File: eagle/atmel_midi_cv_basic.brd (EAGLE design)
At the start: 100 x 80 mm, 46 parts, among them IC1 TL072P, IC2 TL072P, U1 ATMEGA328P_PDIP

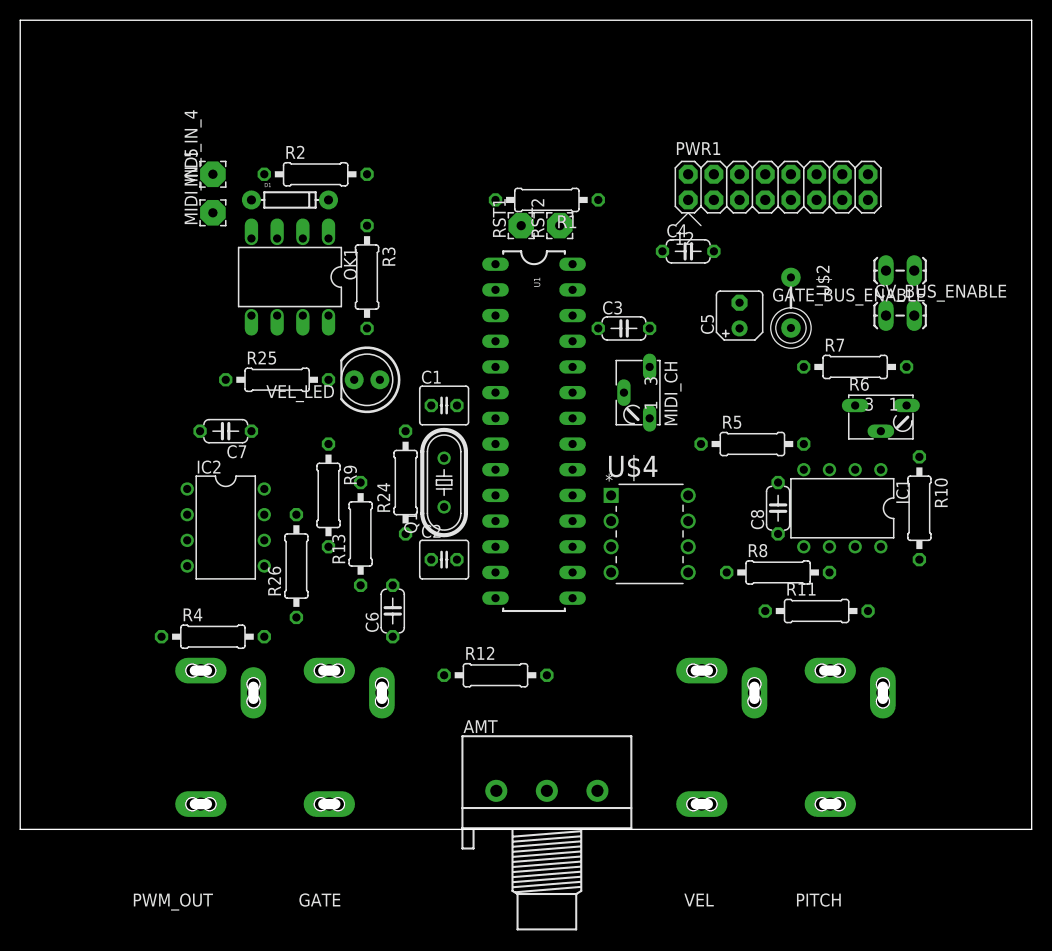
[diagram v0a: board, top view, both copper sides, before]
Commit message: possible route
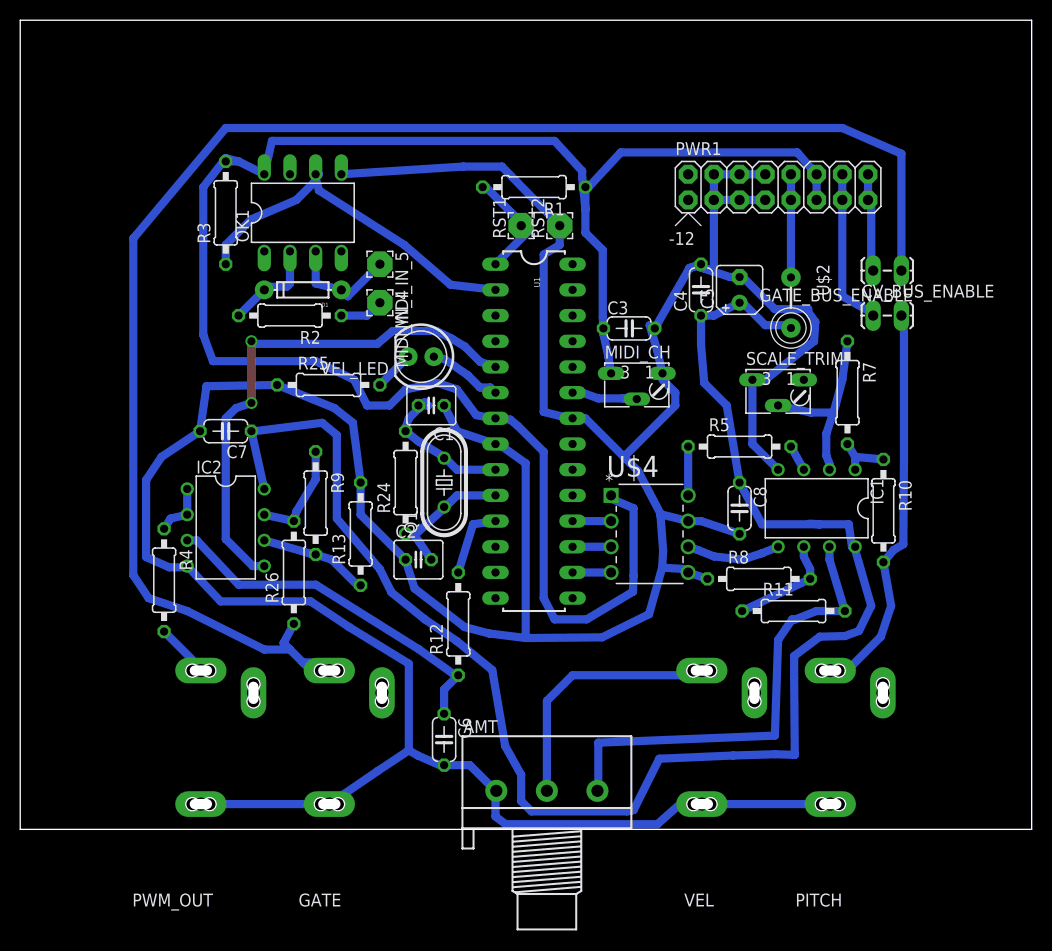
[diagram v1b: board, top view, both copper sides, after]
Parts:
- removed R6: 10k, pot:B64W
- added SCALE_TRIM: 10k, pot:B64W
- moved MIDI_IN_4 20.8 mm to (35.6, 52.1), turned to 270 degrees
- moved MIDI_IN_5 17.3 mm to (35.6, 55.9), turned to 270 degrees
- moved R3 15.3 mm to (20.3, 61.0), turned to 90 degrees
- moved R2 14.2 mm to (26.7, 50.8), turned to 180 degrees
- moved C6 13.7 mm to (41.9, 8.89), turned to 270 degrees
- moved D1 8.98 mm to (27.9, 53.3), turned to 180 degrees
- moved R4 7.38 mm to (14.2, 24.6), turned to 270 degrees
- moved OK1 6.48 mm to (27.9, 61.0), turned to 0 degrees
- moved R12 6.27 mm to (43.3, 20.3), turned to 90 degrees
- moved VEL_LED 5.80 mm to (39.6, 46.7)
- moved R25 5.11 mm to (30.5, 43.9)
- moved C4 4.02 mm to (67.3, 53.3), turned to 90 degrees
- moved C8 3.81 mm to (71.1, 31.8), turned to 270 degrees
- moved R10 3.57 mm to (85.3, 31.5)
- moved R7 2.65 mm to (81.8, 43.2), turned to 270 degrees
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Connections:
- removed net GND: AMT.1, C1.1, C2.1, C3.2, C4.2, C5.-, C6.2, C7.2, C8.2, GATE.P$1, IC1.4, IC2.4, MIDI_CH.E, OK1.5, PITCH.P$1, PWM_OUT.P$1, PWR1.3, PWR1.4, PWR1.5, PWR1.6, PWR1.7, PWR1.8, R13.2, R25.1, R6.E, R8.1, RST2.1, U$4.5, U$4.7, U1.22, U1.8, VEL.P$1
- new net N$29: AMT.1, C1.1, C2.1, C3.2, C4.2, C5.-, C6.2, C7.2, C8.2, GATE.P$1, IC1.4, IC2.4, MIDI_CH.A, OK1.5, PITCH.P$1, PWM_OUT.P$1, PWR1.3, PWR1.4, PWR1.5, PWR1.6, PWR1.7, PWR1.8, R13.2, R25.1, R8.1, RST2.1, SCALE_TRIM.E, U$4.5, U$4.7, U1.22, U1.8, VEL.P$1
- net +5V: now also MIDI_CH.E; no longer MIDI_CH.A
- net N$12: now also SCALE_TRIM.S; no longer R6.S
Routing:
- net N$29: track 0.00 -> 375.6 mm
- net +5V: track 0.00 -> 187.3 mm
- net +12V: track 0.00 -> 159.4 mm
- net N$31: track 0.00 -> 155.0 mm
- net N$22: track 0.00 -> 51.8 mm, vias 0 -> 2
- net N$17: track 0.00 -> 46.2 mm
- net N$9: track 0.00 -> 39.5 mm
- net N$30: track 0.00 -> 36.3 mm
- net N$28: track 0.00 -> 35.7 mm
- net N$51: track 0.00 -> 25.5 mm
- net N$12: track 0.00 -> 18.6 mm
- net N$15: track 0.00 -> 15.8 mm
- net N$4: track 0.00 -> 15.2 mm
- net N$5: track 0.00 -> 13.4 mm
- net N$3: track 0.00 -> 11.2 mm
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
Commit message: routed
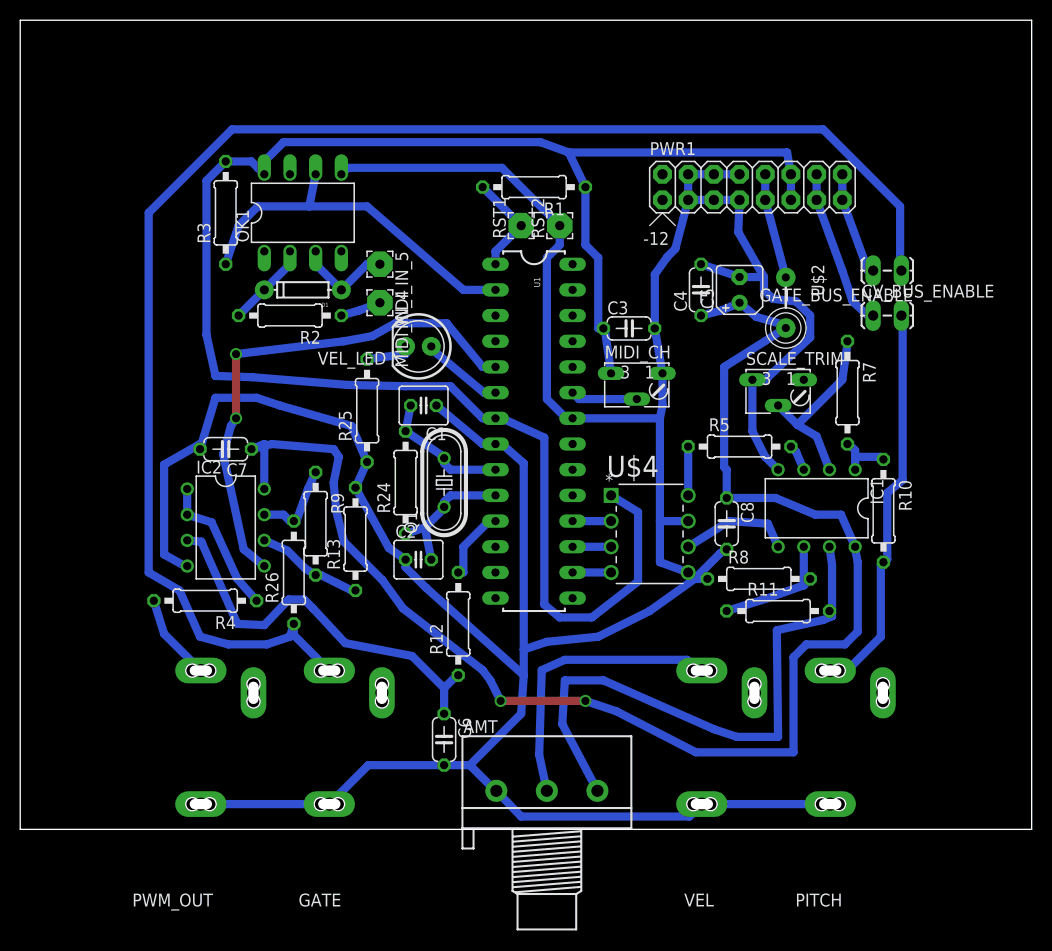
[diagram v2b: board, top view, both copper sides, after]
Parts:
- moved R25 4.58 mm to (34.3, 41.4), turned to 90 degrees
- moved R4 4.54 mm to (18.3, 22.6), turned to 180 degrees
- moved PWR1 2.54 mm to (69.8, 63.5)
- moved R9 2.03 mm to (29.2, 30.2)
- moved C8 1.98 mm to (69.8, 30.2)
- moved C7 1.78 mm to (20.3, 37.6)
- moved R11 1.52 mm to (74.9, 21.6)
- moved VEL_LED 1.05 mm to (39.4, 47.8)
- moved C1 0.76 mm to (39.9, 41.9)
- moved R13 0.72 mm to (33.1, 28.7)
- moved U$2 0.51 mm to (75.7, 52.1)
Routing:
- net N$29: track 375.6 -> 352.0 mm
- net +12V: track 159.4 -> 145.9 mm, vias 0 -> 2
- net N$17: track 46.2 -> 57.6 mm
- net N$23: track 5.43 -> 14.1 mm
- net +5V: track 187.3 -> 179.9 mm
- net N$31: track 155.0 -> 148.0 mm
- net N$28: track 35.7 -> 39.6 mm
- net N$51: track 25.5 -> 28.4 mm
- net N$24: track 5.66 -> 8.57 mm
- net N$4: track 15.2 -> 13.1 mm
- net N$13: track 10.8 -> 12.7 mm
- net N$14: track 9.31 -> 11.1 mm
- net N$16: track 10.4 -> 8.63 mm
- net N$19: track 8.09 -> 6.61 mm
- net N$3: track 11.2 -> 9.72 mm
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
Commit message: new gcode
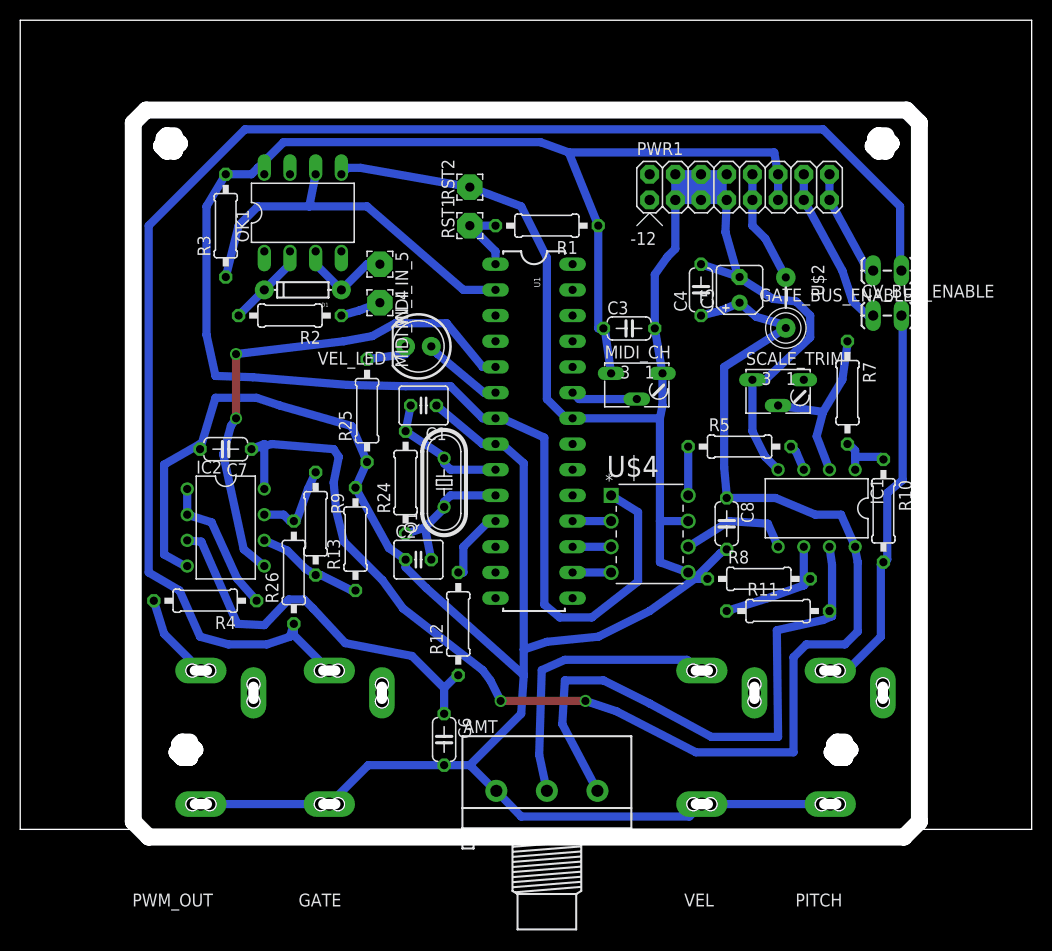
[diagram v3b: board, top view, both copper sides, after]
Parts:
- moved RST2 9.67 mm to (44.5, 63.5)
- moved RST1 5.08 mm to (44.5, 59.7)
- moved R1 4.02 mm to (52.1, 59.7)
- moved R3 1.27 mm to (20.3, 59.7)
- moved PWR1 1.27 mm to (68.6, 63.5)
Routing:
- net N$29: track 352.0 -> 346.9 mm
- net +5V: track 179.9 -> 176.7 mm
- net N$43: track 10.3 -> 7.40 mm
- net N$30: track 36.5 -> 37.7 mm
- net N$11: track 10.5 -> 11.2 mm
- net N$31: track 148.0 -> 147.2 mm
- net N$15: track 15.8 -> 16.3 mm
- net N$1: track 10.5 -> 11.0 mm
- net N$12: track 18.6 -> 18.1 mm
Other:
- board size 100 x 80 mm -> 100 x 80.8 mm

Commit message: layout tweaked
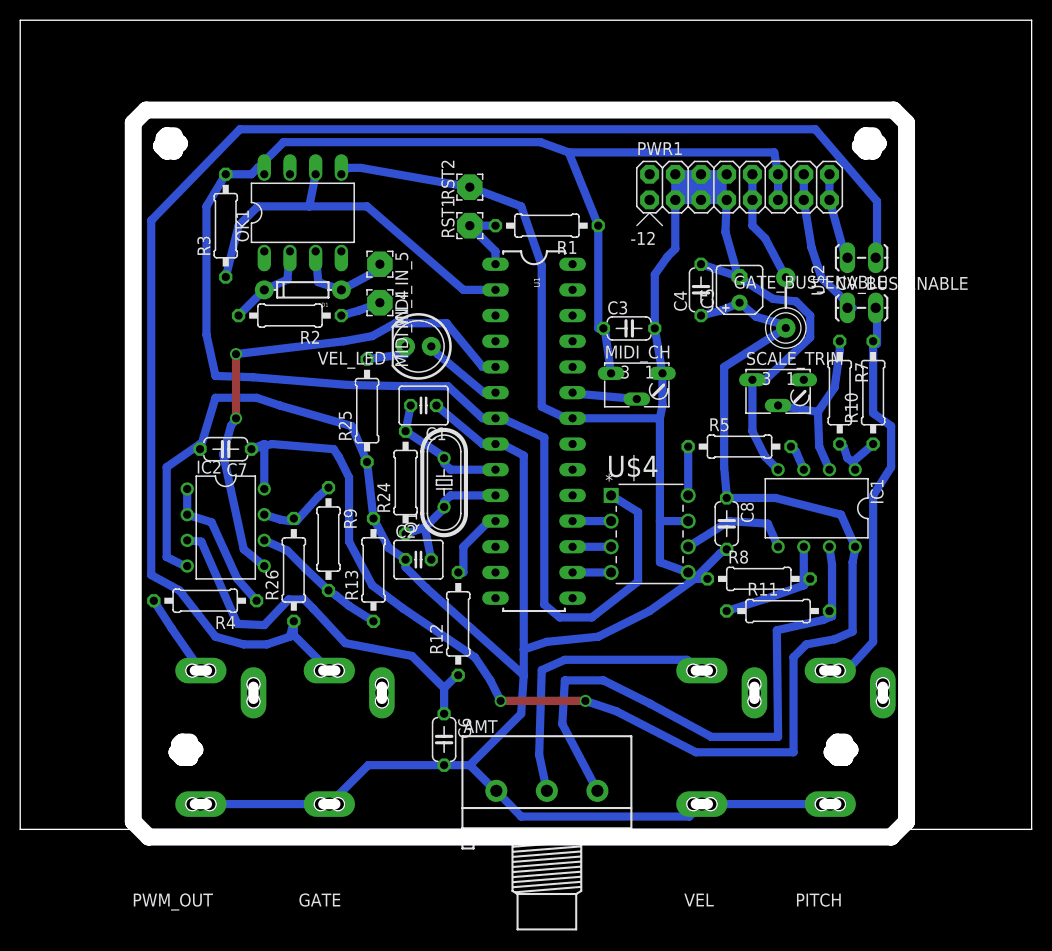
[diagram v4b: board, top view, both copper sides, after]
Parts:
- moved R10 11.7 mm to (84.3, 43.2), turned to 90 degrees
- moved R13 3.53 mm to (34.9, 25.7)
- moved GATE_BUS_ENABLE 2.84 mm to (84.5, 56.5)
- moved CV_BUS_ENABLE 2.65 mm to (81.9, 51.6)
- moved R9 1.98 mm to (30.5, 28.7)
- moved R7 0.76 mm to (81.0, 43.2)
- moved R26 0.25 mm to (27.1, 25.7)
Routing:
- net N$9: track 39.3 -> 42.8 mm
- net N$31: track 147.2 -> 144.0 mm
- net N$10: track 10.5 -> 13.6 mm
- net N$1: track 11.0 -> 8.57 mm
- net N$15: track 16.3 -> 15.2 mm
- net +12V: track 145.8 -> 144.9 mm
- net N$12: track 18.1 -> 17.5 mm
- net N$16: track 8.63 -> 8.03 mm
- net N$3: track 9.72 -> 10.3 mm
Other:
- outline, holes or cut-outs redrawn
